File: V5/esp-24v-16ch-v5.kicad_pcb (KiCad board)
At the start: 4 copper layers, 128 x 67.8 mm, 327 parts, among them J1 KF250-3.5-8P-1, J2 GNDIO, J3 KF250-3.5-8P-1, J4 KF250-3.5-8P-1, J5 KF250-3.5-8P-1, J6 VIN, J7 USB_C_Receptacle_USB2.0, J8 ETHERNET, J9 SENSORS, Q1 WPM2015-3/TR, Q10 MMBT2222A, Q11 MMBT2222A, Q12 MMBT2222A, Q13 MMBT2222A, Q14 MMBT2222A, Q15 MMBT2222A, Q16 MMBT2222A, Q17 MMBT2222A, Q18 MMBT2222A, Q19 MMBT2222A, Q2 MMUN2211LT3G, Q3 UMH3N, Q4 MMBT2222A, Q5 MMBT2222A, Q6 MMBT2222A, Q7 MMBT2222A, Q8 MMBT2222A, Q9 MMBT2222A, SW1 RESET, SW2 1WIRE_SEL, U1 SY8089A1AAC, U10 OR-3H7-4, U11 OR-3H7-4, U12 OR-3H7-4, U13 OR-3H7-4, U2 TX4138, U3 CH340K, U4 ESP32-WROOM-32UE-N16, U5 LAN8710A, U6 MCP23008-xSS, U7 MCP23008-xSS, U8 MCP23017_SS, U9 DS2482S-100

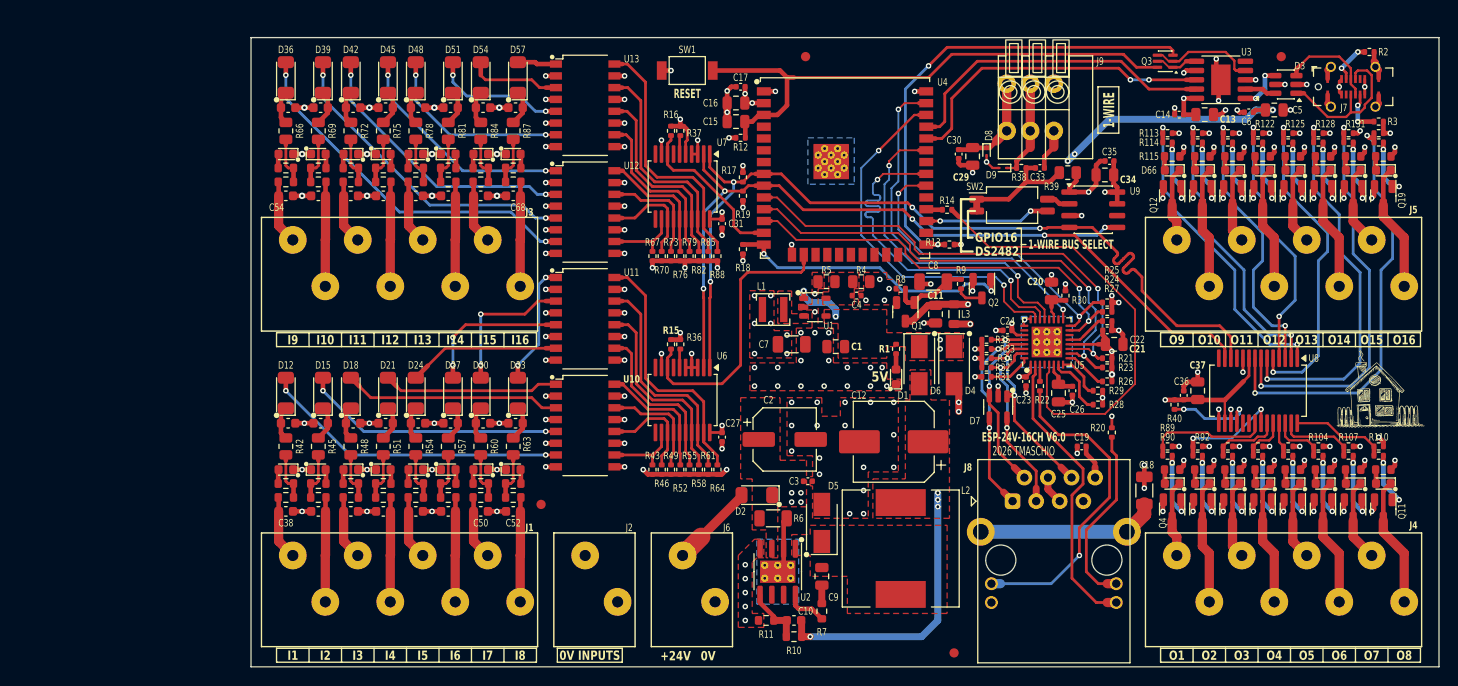
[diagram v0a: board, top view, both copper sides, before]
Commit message: V6 is up
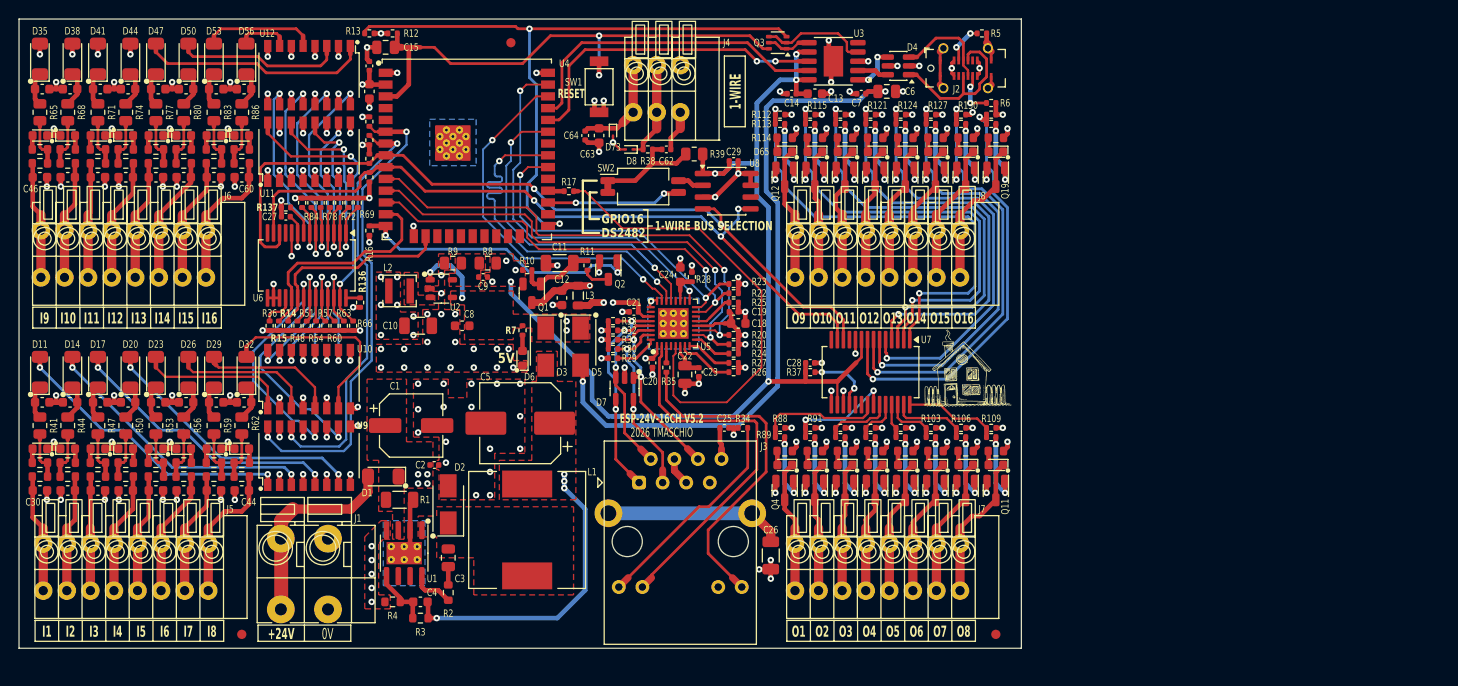
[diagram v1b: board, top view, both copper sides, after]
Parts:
- removed the C1 at (152.8, 99.6)
- removed the C11 at (163.5, 96.1)
- removed the C20 at (176.0, 93.6)
- removed the C21 at (182.8, 99.3)
- removed the C29 at (167.5, 79.1)
- removed the C31 at (140.5, 86.3)
- removed the C34 at (181.8, 81.1)
- removed the C37 at (191.8, 104.3)
- removed FID4: Fiducial, Fiducial:Fiducial_1mm_Mask2mm
- removed the J2 at (127.5, 124.6)
- removed the J4 at (201.8, 124.6)
- removed the R16 at (135.0, 76.3)
- removed the R37 at (136.0, 76.3)
- removed the R43 at (133.0, 112.8)
- removed the R46 at (134.0, 112.8)
- removed the R49 at (135.0, 112.8)
- removed the R52 at (136.0, 112.8)
- removed the R55 at (137.0, 112.8)
- removed the R58 at (138.0, 112.8)
- removed the R61 at (139.0, 112.8)
- removed the R64 at (140.0, 112.8)
- removed the R67 at (133.0, 89.8)
- removed the R70 at (134.0, 89.8)
- removed the R73 at (135.0, 89.8)
- removed the R76 at (136.0, 89.8)
- removed the R79 at (137.0, 89.8)
- removed the R82 at (138.0, 89.8)
- removed the R85 at (139.0, 89.8)
- removed the R88 at (140.0, 89.8)
- removed the U7 at (136.3, 82.3)
- added C12: 10uF/10V, Tales:C_0603_1608Metric, F.Cu at (123.3, 94.3)
- added C18: 10uF/10V, Tales:C_0603_1608Metric, F.Cu at (142.3, 97.1)
- added C24: 10uF/10V, Tales:C_0603_1608Metric, F.Cu at (136.0, 91.8)
- added C63: 10uF/10V, Tales:C_0603_1608Metric, F.Cu at (127.3, 76.8)
- added C8: 10uF/10V, Tales:C_0603_1608Metric, F.Cu at (112.5, 97.3)
- added J7: DB141V-2.54-8P, Tales:TerminalBlock_Dibo_DB141V-2.54-8P_1x08_P2.54mm_Vertical, F.Cu at (157.3, 123.3)
- added R136: 10k, Tales:R_0402_1005Metric, F.Cu at (101.5, 94.8)
- added R137: 10k, Tales:R_0402_1005Metric, F.Cu at (93.5, 84.6)
- added R15: 2k2, Tales:R_0402_1005Metric, F.Cu at (92.8, 97.3)
- added R42: 2k2, Tales:R_0402_1005Metric, F.Cu at (102.5, 75.3)
- added R45: 2k2, Tales:R_0402_1005Metric, F.Cu at (102.5, 77.3)
- added R48: 2k2, Tales:R_0402_1005Metric, F.Cu at (94.8, 97.3)
- added R51: 2k2, Tales:R_0402_1005Metric, F.Cu at (95.8, 97.3)
- added R54: 2k2, Tales:R_0402_1005Metric, F.Cu at (96.8, 97.3)
- added R57: 2k2, Tales:R_0402_1005Metric, F.Cu at (97.8, 97.3)
- added R60: 2k2, Tales:R_0402_1005Metric, F.Cu at (98.8, 97.3)
- added R63: 2k2, Tales:R_0402_1005Metric, F.Cu at (99.8, 97.3)
- added R66: 2k2, Tales:R_0402_1005Metric, F.Cu at (100.8, 97.3)
- added R69: 2k2, Tales:R_0402_1005Metric, F.Cu at (101.3, 84.1)
- added R72: 2k2, Tales:R_0402_1005Metric, F.Cu at (100.3, 84.1)
- added R75: 2k2, Tales:R_0402_1005Metric, F.Cu at (99.3, 84.1)
- added R78: 2k2, Tales:R_0402_1005Metric, F.Cu at (98.3, 84.1)
- added R81: 2k2, Tales:R_0402_1005Metric, F.Cu at (97.3, 84.1)
- added R84: 2k2, Tales:R_0402_1005Metric, F.Cu at (96.3, 84.1)
- added R87: 2k2, Tales:R_0402_1005Metric, F.Cu at (95.3, 84.1)
- C13, C16: value 10uF/25V -> 10uF/10V; footprint Tales:C_0805_2012Metric -> Tales:C_0603_1608Metric
- J1: value KF250-3.5-8P-1 -> VIN; footprint Tales:TerminalBlock_Wago_250-208_1x08_P3.5mm_45Degree -> Tales:TerminalBlock_Dibo_DB142V-5.08-2P_1x02_P5.08mm_Vertical
- J3: value KF250-3.5-8P-1 -> ETHERNET; footprint Tales:TerminalBlock_Wago_250-208_1x08_P3.5mm_45Degree -> Tales:RJ45_HanRun_HR911105A
- J5: value KF250-3.5-8P-1 -> DB141V-2.54-8P; footprint Tales:TerminalBlock_Wago_250-208_1x08_P3.5mm_45Degree -> Tales:TerminalBlock_Dibo_DB141V-2.54-8P_1x08_P2.54mm_Vertical
- J6: value VIN -> DB141V-2.54-8P; footprint Tales:TerminalBlock_Wago_250-202_1x02_P3.5mm_45Degree -> Tales:TerminalBlock_Dibo_DB141V-2.54-8P_1x08_P2.54mm_Vertical
- J8: value ETHERNET -> DB141V-2.54-8P; footprint Tales:RJ45_HanRun_HR915340A -> Tales:TerminalBlock_Dibo_DB141V-2.54-8P_1x08_P2.54mm_Vertical
- U6: value MCP23008-xSS -> MCP23017_SS; footprint Package_SO:SSOP-20_5.3x7.2mm_P0.65mm -> Package_SO:SSOP-28_5.3x10.2mm_P0.65mm
- moved J5 129.7 mm to (76.3, 123.3)
- moved J6 71.2 mm to (76.0, 89.6)
- moved R13 66.5 mm to (102.5, 65.8)
- moved C27 52.7 mm to (93.5, 85.6), turned to 180 degrees
- moved Ref** 44.6 mm to (166.5, 106.1)
- moved R36 44.3 mm to (91.8, 97.3), turned to 90 degrees
- moved U6 43.0 mm to (95.8, 90.8)
- moved J3 42.1 mm to (136.0, 120.6)
- moved C13 42.1 mm to (150.5, 72.3)
- moved C14 41.8 mm to (148.0, 72.3)
- moved C6 41.8 mm to (158.3, 72.1)
- moved C7 41.8 mm to (155.5, 72.3)
- moved D4 41.8 mm to (159.5, 69.3)
- moved D57 41.8 mm to (147.3, 112.3)
- moved D58 41.8 mm to (150.5, 112.3)
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- renumbered C2 to C1, C7 to C10, C8 to C11, C22 to C19, C3 to C2, C23 to C20, C24 to C21, C25 to C22, C26 to C23, C19 to C25, C18 to C26, C36 to C28, C35 to C29, C9 to C3, C38 to C30, C39 to C31, C40 to C32, C41 to C33, C42 to C34, C43 to C35, C44 to C36, C45 to C37, C46 to C38, C47 to C39, C10 to C4, C48 to C40, C49 to C41, C50 to C42, C51 to C43, C52 to C44, C53 to C45, C54 to C46, C55 to C47, C56 to C48, C57 to C49, C12 to C5, C58 to C50, C59 to C51, C60 to C52, C61 to C53, C62 to C54, C63 to C55, C64 to C56, C65 to C57, C66 to C58, C67 to C59, C5 to C6, C68 to C60, C69 to C61, C33 to C62, C30 to C64, C6 to C7, C4 to C9, D2 to D1, D11 to D10, D12 to D11, D14 to D13, D15 to D14, D17 to D16, D18 to D17, D20 to D19, D5 to D2, D21 to D20, D23 to D22, D24 to D23, D26 to D25, D27 to D26, D29 to D28, D30 to D29, D6 to D3, D32 to D31, D33 to D32, D35 to D34, D36 to D35, D38 to D37, D39 to D38, D3 to D4, D41 to D40, D42 to D41, D44 to D43, D45 to D44, D47 to D46, D48 to D47, D50 to D49, D4 to D5, D51 to D50, D53 to D52, D54 to D53, D56 to D55, D57 to D56, D58 to D57, D59 to D58, D60 to D59, D1 to D6, D61 to D60, D62 to D61, D63 to D62, D64 to D63, D65 to D64, D66 to D65, D67 to D66, D68 to D67, D69 to D68, D70 to D69, D71 to D70, D72 to D71, D73 to D72, D8 to D73, D9 to D8, J7 to J2, J9 to J4, L2 to L1, L1 to L2, R6 to R1, R8 to R10, R101 to R100, R102 to R101, R103 to R102, R104 to R103, R105 to R104, R106 to R105, R107 to R106, R108 to R107, R109 to R108, R110 to R109, R9 to R11, R111 to R110, R112 to R111, R113 to R112, R114 to R113, R115 to R114, R116 to R115, R117 to R116, R118 to R117, R119 to R118, R120 to R119, R121 to R120, R122 to R121, R123 to R122, R124 to R123, R125 to R124, R126 to R125, R127 to R126, R128 to R127, R129 to R128, R130 to R129, R131 to R130, R132 to R131, R133 to R132, R134 to R133, R135 to R134, R136 to R135, R15 to R14, R18 to R16, R14 to R17, R17 to R18, R7 to R2, R21 to R20, R23 to R21, R24 to R22, R25 to R23, R26 to R24, R27 to R25, R28 to R26, R29 to R27, R30 to R28, R31 to R29, R10 to R3, R32 to R30, R34 to R31, R33 to R32, R35 to R33, R20 to R34, R22 to R35, R40 to R37, R11 to R4, R41 to R40, R42 to R41, R44 to R43, R45 to R44, R47 to R46, R48 to R47, R50 to R49, R2 to R5, R51 to R50, R53 to R52, R54 to R53, R56 to R55, R57 to R56, R59 to R58, R60 to R59, R3 to R6, R62 to R61, R63 to R62, R65 to R64, R66 to R65, R68 to R67, R69 to R68, R1 to R7, R71 to R70, R72 to R71, R74 to R73, R75 to R74, R77 to R76, R78 to R77, R80 to R79, R4 to R8, R81 to R80, R83 to R82, R84 to R83, R86 to R85, R87 to R86, R89 to R88, R90 to R89, R5 to R9, R91 to R90, R92 to R91, R93 to R92, R94 to R93, R95 to R94, R96 to R95, R97 to R96, R98 to R97, R99 to R98, R100 to R99, U2 to U1, U11 to U10, U12 to U11, U13 to U12, U1 to U2, U8 to U7, U9 to U8, U10 to U9
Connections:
- C30 pad 2: GNDIO -> GND
- C31 pad 2: GNDIO -> GND
- C32 pad 2: GNDIO -> GND
- C33 pad 2: GNDIO -> GND
- C34 pad 2: GNDIO -> GND
- C35 pad 2: GNDIO -> GND
- C36 pad 2: GNDIO -> GND
- C37 pad 2: GNDIO -> GND
- C38 pad 2: GNDIO -> GND
- C39 pad 2: GNDIO -> GND
- C40 pad 2: GNDIO -> GND
- C41 pad 2: GNDIO -> GND
- C42 pad 2: GNDIO -> GND
- C43 pad 2: GNDIO -> GND
- C44 pad 2: GNDIO -> GND
- C45 pad 2: GNDIO -> GND
- C46 pad 2: GNDIO -> GND
- C47 pad 2: GNDIO -> GND
- C48 pad 2: GNDIO -> GND
- C49 pad 2: GNDIO -> GND
- C50 pad 2: GNDIO -> GND
- C51 pad 2: GNDIO -> GND
- C52 pad 2: GNDIO -> GND
- C53 pad 2: GNDIO -> GND
- C54 pad 2: GNDIO -> GND
- C55 pad 2: GNDIO -> GND
- C56 pad 2: GNDIO -> GND
- C57 pad 2: GNDIO -> GND
- C58 pad 2: GNDIO -> GND
- C59 pad 2: GNDIO -> GND
- C60 pad 2: GNDIO -> GND
- C61 pad 2: GNDIO -> GND
- D10 pad 1: GNDIO -> GND
- D13 pad 1: GNDIO -> GND
- D16 pad 1: GNDIO -> GND
- D19 pad 1: GNDIO -> GND
- D22 pad 1: GNDIO -> GND
- D25 pad 1: GNDIO -> GND
- D28 pad 1: GNDIO -> GND
- D31 pad 1: GNDIO -> GND
- D34 pad 1: GNDIO -> GND
- D37 pad 1: GNDIO -> GND
- D40 pad 1: GNDIO -> GND
- D43 pad 1: GNDIO -> GND
- D46 pad 1: GNDIO -> GND
- D49 pad 1: GNDIO -> GND
- D52 pad 1: GNDIO -> GND
- D55 pad 1: GNDIO -> GND
- J1 pad 1: /IN1 -> /Power/+24VIN
- J1 pad 2: /IN2 -> GND
- J3 pad 1: /IN9 -> /LAN/ETHTXD+
- J3 pad 2: /IN10 -> /LAN/ETHTXD-
- J3 pad 3: /IN11 -> /LAN/ETHRXD+
- J3 pad 4: /IN12 -> +3V3A
- J3 pad 5: /IN13 -> +3V3A
- J3 pad 6: /IN14 -> /LAN/ETHRXD-
- J3 pad 7: /IN15 -> unconnected-(J3-NC-Pad7)
- J3 pad 8: /IN16 -> GND
- J5 pad 1: /OUT9 -> /IN1
- J5 pad 2: /OUT10 -> /IN2
- J5 pad 3: /OUT11 -> /IN3
- J5 pad 4: /OUT12 -> /IN4
- J5 pad 5: /OUT13 -> /IN5
- J5 pad 6: /OUT14 -> /IN6
- J5 pad 7: /OUT15 -> /IN7
- J5 pad 8: /OUT16 -> /IN8
- J6 pad 1: /Power/+24VIN -> /IN9
- J6 pad 2: GND -> /IN10
- J8 pad 1: /LAN/ETHTXD+ -> /OUT9
- J8 pad 2: /LAN/ETHTXD- -> /OUT10
- J8 pad 3: /LAN/ETHRXD+ -> /OUT11
- J8 pad 4: +3V3A -> /OUT12
- J8 pad 5: +3V3A -> /OUT13
- J8 pad 6: /LAN/ETHRXD- -> /OUT14
- J8 pad 7: unconnected-(J8-NC-Pad7) -> /OUT15
- J8 pad 8: GND -> /OUT16
- R14 pad 2: /I2C Devices/MCPIN1INT -> /I2C Devices/MCPININTA
- R34 pad 1: +3V3LAN -> +3V3A
- R36 pad 2: /I2C Devices/MCPINN1RST -> /I2C Devices/MCPINNRST
- U10 pad 1: /Input 8/INOPTO -> /Input 5/INOPTO
- U10 pad 10: /INPUT5 -> /INPUT8
- U10 pad 12: /INPUT6 -> /INPUT7
- U10 pad 14: /INPUT7 -> /INPUT6
- U10 pad 16: /INPUT8 -> /INPUT5
- U10 pad 2: GNDIO -> GND
- U10 pad 3: /Input 7/INOPTO -> /Input 6/INOPTO
- U10 pad 4: GNDIO -> GND
- U10 pad 5: /Input 6/INOPTO -> /Input 7/INOPTO
- U10 pad 6: GNDIO -> GND
- U10 pad 7: /Input 5/INOPTO -> /Input 8/INOPTO
- U10 pad 8: GNDIO -> GND
- U11 pad 1: /Input 12/INOPTO -> /Input 9/INOPTO
- U11 pad 10: /INPUT9 -> /INPUT12
- U11 pad 12: /INPUT10 -> /INPUT11
- U11 pad 14: /INPUT11 -> /INPUT10
- U11 pad 16: /INPUT12 -> /INPUT9
- U11 pad 2: GNDIO -> GND
- U11 pad 3: /Input 11/INOPTO -> /Input 10/INOPTO
- U11 pad 4: GNDIO -> GND
- U11 pad 5: /Input 10/INOPTO -> /Input 11/INOPTO
- U11 pad 6: GNDIO -> GND
- U11 pad 7: /Input 9/INOPTO -> /Input 12/INOPTO
- U11 pad 8: GNDIO -> GND
- U12 pad 1: /Input 16/INOPTO -> /Input 13/INOPTO
- U12 pad 10: /INPUT13 -> /INPUT16
- U12 pad 12: /INPUT14 -> /INPUT15
- U12 pad 14: /INPUT15 -> /INPUT14
- U12 pad 16: /INPUT16 -> /INPUT13
- U12 pad 2: GNDIO -> GND
- U12 pad 3: /Input 15/INOPTO -> /Input 14/INOPTO
- U12 pad 4: GNDIO -> GND
- U12 pad 5: /Input 14/INOPTO -> /Input 15/INOPTO
- U12 pad 6: GNDIO -> GND
- U12 pad 7: /Input 13/INOPTO -> /Input 16/INOPTO
- U12 pad 8: GNDIO -> GND
- U4 pad 13: /I2C Devices/MCPIN2INT -> /I2C Devices/MCPININTB
- U4 pad 16: /I2C Devices/MCPIN1INT -> /I2C Devices/MCPININTA
- U4 pad 6: unconnected-(U4-IO34-Pad6) -> /INPUT1
- U4 pad 7: unconnected-(U4-IO35-Pad7) -> /INPUT2
- U6 pad 1: /I2C Devices/I2CSCL -> /INPUT10
- U6 pad 10: unconnected-(U6-NC-Pad10) -> GND
- U6 pad 12: /INPUT1 -> /I2C Devices/I2CSCL
- U6 pad 13: /INPUT2 -> /I2C Devices/I2CSDA
- U6 pad 14: /INPUT3 -> unconnected-(U6-NC-Pad14)
- U6 pad 15: /INPUT4 -> GND
- U6 pad 16: /INPUT5 -> GND
- U6 pad 17: /INPUT6 -> GND
- U6 pad 18: /INPUT7 -> /I2C Devices/MCPINNRST
- U6 pad 19: /INPUT8 -> /I2C Devices/MCPININTB
- U6 pad 2: /I2C Devices/I2CSDA -> /INPUT11
- U6 pad 20: +3V3 -> /I2C Devices/MCPININTA
- U6 pad 3: GND -> /INPUT12
- U6 pad 4: GND -> /INPUT13
- U6 pad 5: GND -> /INPUT14
- U6 pad 6: /I2C Devices/MCPINN1RST -> /INPUT15
- U6 pad 7: unconnected-(U6-NC-Pad7) -> /INPUT16
- U6 pad 8: /I2C Devices/MCPIN1INT -> /I2C Devices/GPB7
- U6 pad 9: GND -> +3V3
- U9 pad 1: /Input 4/INOPTO -> /Input 1/INOPTO
- U9 pad 10: /INPUT1 -> /INPUT4
- U9 pad 12: /INPUT2 -> /INPUT3
- U9 pad 14: /INPUT3 -> /INPUT2
- U9 pad 16: /INPUT4 -> /INPUT1
- U9 pad 2: GNDIO -> GND
- U9 pad 3: /Input 3/INOPTO -> /Input 2/INOPTO
- U9 pad 4: GNDIO -> GND
- U9 pad 5: /Input 2/INOPTO -> /Input 3/INOPTO
- U9 pad 6: GNDIO -> GND
- U9 pad 7: /Input 1/INOPTO -> /Input 4/INOPTO
- U9 pad 8: GNDIO -> GND
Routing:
- net +3V3: track 73.7 -> 143.3 mm, vias 31 -> 25
- net GND: track 135.4 -> 204.8 mm, vias 131 -> 180
- net GNDIO: track 64.2 -> 0.00 mm, vias 40 -> 0
- net /INPUT1: track 8.07 -> 52.2 mm, vias 0 -> 2
- net /INPUT2: track 11.3 -> 46.1 mm, vias 0 -> 2
- net /I2C Devices/MCPIN1INT: track 30.3 -> 0.00 mm
- net /I2C Devices/MCPININTB: track 0.00 -> 23.9 mm
- net /INPUT9: track 8.07 -> 30.6 mm, vias 0 -> 2
- net /I2C Devices/MCPININTA: track 0.00 -> 22.1 mm
- net /MCU/ESPPROG: track 52.4 -> 71.9 mm
- net /I2C Devices/MCPIN2INT: track 17.7 -> 0.00 mm
- net /OUTPUT12: track 29.1 -> 46.4 mm
- net /OUTPUT10: track 32.2 -> 49.5 mm
- net /OUTPUT11: track 30.9 -> 47.9 mm
- net /OUTPUT9: track 34.2 -> 51.0 mm
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- removed copper zone on In1.Cu, net GNDIO
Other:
- board size 128 x 67.8 mm -> 108 x 67.8 mm
- board text added: "1-WIRE BUS SELECTION"
- board text added: "ESP-24V-16CH V5.2"
- board text added: "SUPORTES PCI METALTEX SP7 1x pé macho 9 mm 1x pé fêmea 9 mm 2x espaçadores 45 mm Comprimento total 108 mm Largura da placa 67,8 mm"
- board text removed: "0V INPUTS"
- board text removed: "1-WIRE BUS SELECT"
- board text removed: "ESP-24V-16CH V6.0"
- board text removed: "SUPORTES PCI METALTEX SP7 1x pé macho 9 mm 1x pé fêmea 9 mm 2x espaçadores 45 mm 1x espaçador 20 mm Comprimento total 128 mm Largura da placa 67,8 mm"
